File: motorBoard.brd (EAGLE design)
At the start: 97.8 x 68.6 mm, 71 parts, among them J1 TE-TERM-BLOCK, J2 TE-TERM-BLOCK

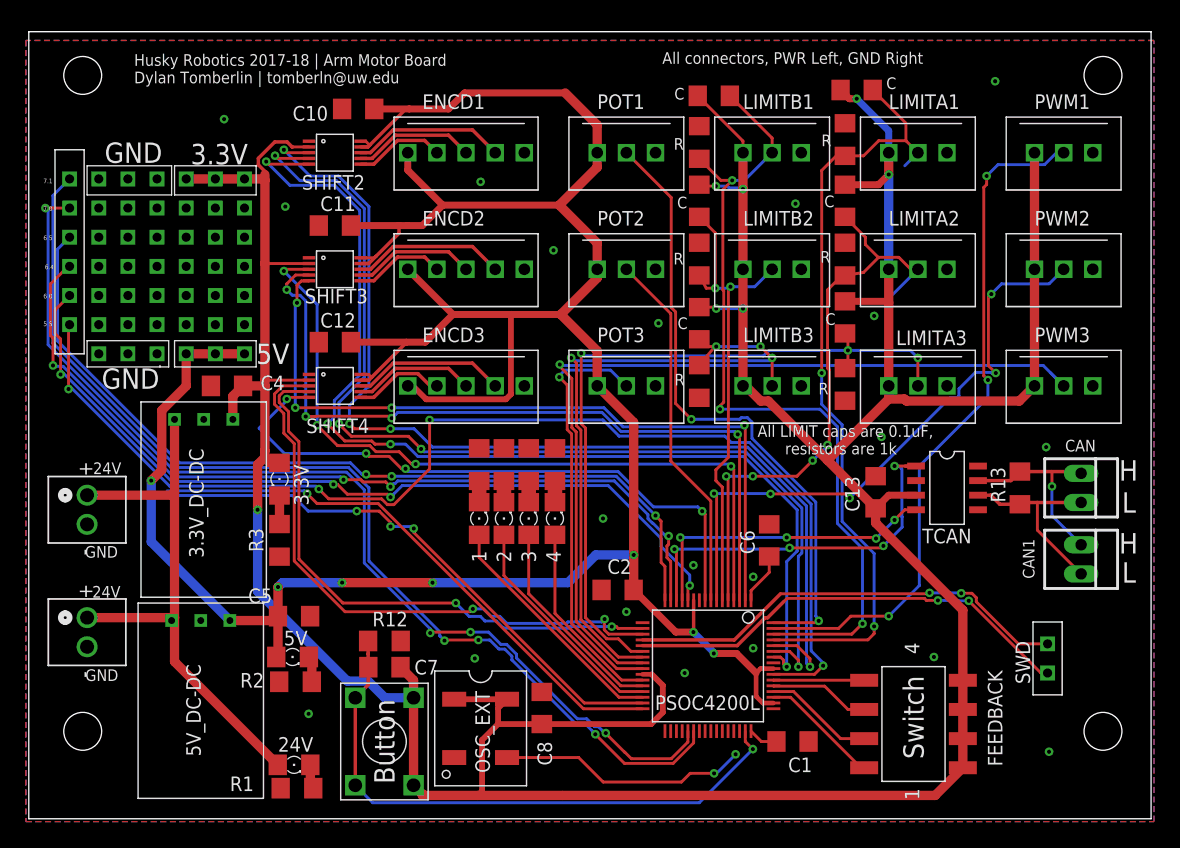
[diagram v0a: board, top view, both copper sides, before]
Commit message: Made changes for Bay Area Circuits DFM
Re-Zipped
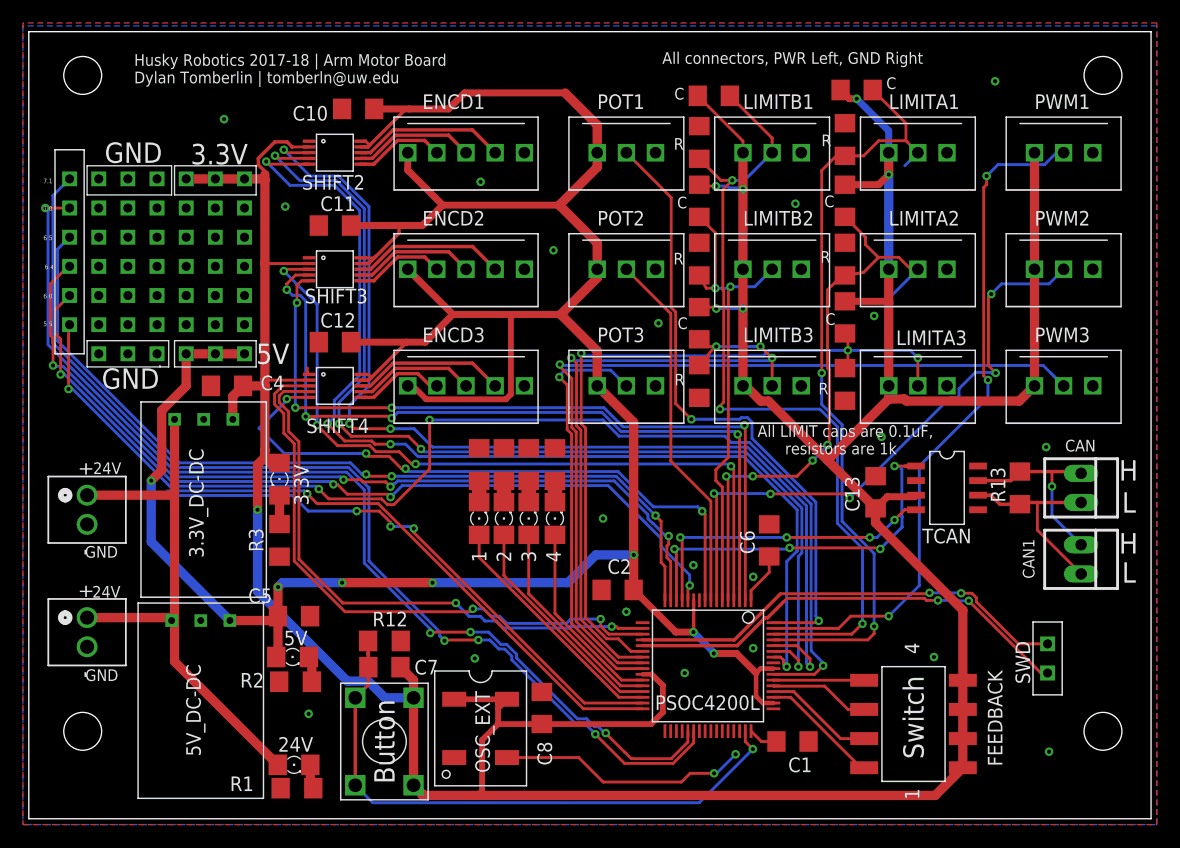
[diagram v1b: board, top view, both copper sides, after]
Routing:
- net GNDA: track 0.00 -> 0.63 mm
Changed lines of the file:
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@@
 <setting verticaltext="up"/>
 </settings>
-<grid distance="0.000000123031" unitdist="inch" unit="inch" style="lines" multiple="1" display="no" altdistance="0.125" altunitdist="inch" altunit="inch"/>
+<grid distance="10" unitdist="mil" unit="mil" style="dots" multiple="1" display="yes" altdistance="0.125" altunitdist="inch" altunit="inch"/>
 <layers>
 <layer number="1" name="Top" color="4" fill="1" visible="yes" active="yes"/>
@@
 <via x="56.7744" y="24.511" extent="1-16" drill="0.35"/>
 <via x="75.438" y="26.035" extent="1-16" drill="0.35"/>
-<wire x1="73.822940625" y1="24.419940625" x2="75.438" y2="26.035" width="0.254" layer="16"/>
 <wire x1="75.438" y1="26.035" x2="76.327" y2="26.924" width="0.254" layer="1"/>
 <wire x1="76.327" y1="26.924" x2="77.31" y2="26.924" width="0.254" layer="1"/>
 <wire x1="56.7744" y1="24.511" x2="66.04" y2="24.511" width="0.254" layer="16"/>
 <via x="66.04" y="24.511" extent="1-16" drill="0.35"/>
-<wire x1="73.73188125" y1="24.511" x2="66.04" y2="24.511" width="0.254" layer="1"/>
-<wire x1="73.73188125" y1="24.511" x2="73.822940625" y2="24.419940625" width="0.254" layer="1"/>
-<via x="73.822940625" y="24.419940625" extent="1-16" drill="0.35"/>
+<wire x1="75.438" y1="26.035" x2="73.914" y2="24.511" width="0.254" layer="16"/>
+<wire x1="73.914" y1="24.511" x2="73.279" y2="24.511" width="0.254" layer="16"/>
+<via x="73.279" y="24.511" extent="1-16" drill="0.35"/>
+<wire x1="73.279" y1="24.511" x2="66.04" y2="24.511" width="0.254" layer="1"/>
 </signal>
 <signal name="CANTX">
@@
 <wire x1="66.1868" y1="23.495" x2="66.294" y2="23.6022" width="0.254" layer="16"/>
 <via x="66.294" y="23.6022" extent="1-16" drill="0.35"/>
-<wire x1="66.294" y1="23.6022" x2="74.29044375" y2="23.6022" width="0.254" layer="1"/>
-<wire x1="74.29044375" y1="23.6022" x2="74.4655625" y2="23.77731875" width="0.254" layer="1"/>
-<via x="74.4655625" y="23.77731875" extent="1-16" drill="0.35"/>
-<wire x1="74.4655625" y1="23.77731875" x2="76.0956" y2="25.40735625" width="0.254" layer="16"/>
 <wire x1="76.0956" y1="25.40735625" x2="76.0956" y2="26.3073875" width="0.254" layer="16"/>
 <wire x1="76.327" y1="30.734" x2="77.31" y2="30.734" width="0.254" layer="1"/>
@@
 <via x="75.438" y="30.734" extent="1-16" drill="0.35"/>
 <wire x1="75.438" y1="30.734" x2="77.31" y2="30.734" width="0.254" layer="1"/>
+<wire x1="66.294" y1="23.6022" x2="74.1017875" y2="23.6022" width="0.254" layer="1"/>
+<wire x1="74.1017875" y1="23.6022" x2="74.19285" y2="23.5111375" width="0.254" layer="1"/>
+<via x="74.19285" y="23.5111375" extent="1-16" drill="0.35"/>
+<wire x1="74.19285" y1="23.5111375" x2="76.08906875" y2="25.40735625" width="0.254" layer="16"/>
+<wire x1="76.08906875" y1="25.40735625" x2="76.0956" y2="25.40735625" width="0.254" layer="16"/>
 </signal>
 <signal name="+5V">
@@
 <via x="52.07" y="18.034" extent="1-16" drill="0.35"/>
 <via x="24.384" y="9.144" extent="1-16" drill="0.35"/>
-<polygon width="0.1524" layer="1">
-<vertex x="-0.254" y="-0.254"/>
-<vertex x="98.044" y="-0.254"/>
-<vertex x="98.044" y="67.818"/>
-<vertex x="-0.254" y="67.818"/>
-</polygon>
-<polygon width="0.1524" layer="16">
-<vertex x="-0.254" y="-0.254"/>
-<vertex x="98.044" y="-0.254"/>
-<vertex x="98.044" y="67.818"/>
-<vertex x="-0.254" y="67.818"/>
-</polygon>
 <contactref element="J1" pad="R"/>
 <contactref element="J2" pad="R"/>
@@
 <contactref element="R14" pad="1"/>
 <contactref element="R15" pad="1"/>
+<wire x1="24.42" y1="38.719" x2="24.2703375" y2="38.8686625" width="0.254" layer="1"/>
+<wire x1="24.2703375" y1="38.8686625" x2="24.2703375" y2="39.28686875" width="0.254" layer="1"/>
+<polygon width="0.1524" layer="1">
+<vertex x="-0.508" y="-0.508"/>
+<vertex x="98.298" y="-0.508"/>
+<vertex x="98.298" y="69.342"/>
+<vertex x="-0.508" y="69.342"/>
+</polygon>
+<polygon width="0.1524" layer="16">
+<vertex x="-0.254" y="-0.508"/>
+<vertex x="98.298" y="-0.508"/>
+<vertex x="98.298" y="69.088"/>
+<vertex x="-0.508" y="69.088"/>
+<vertex x="-0.508" y="-0.508"/>
+</polygon>
 </signal>
 <signal name="+3V3">
@@
 <wire x1="54.2817375" y1="12.585" x2="55.245" y2="11.6217375" width="0.508" layer="1"/>
 <wire x1="53.482" y1="12.585" x2="54.2817375" y2="12.585" width="0.4064" layer="1"/>
-<wire x1="73.787" y1="27.048" x2="74.933" y2="28.194" width="0.6096" layer="1"/>
-<wire x1="74.933" y1="28.194" x2="77.31" y2="28.194" width="0.6096" layer="1"/>
 <wire x1="22.995" y1="58.539" x2="24.42" y2="58.539" width="0.254" layer="1"/>
 <wire x1="20.5640125" y1="31.4860125" x2="20.5640125" y2="32.05911875" width="0.8128" layer="1"/>
@@
 <wire x1="71.12" y1="45.088" x2="74.8" y2="45.088" width="0.6096" layer="1"/>
 <wire x1="74.8" y1="45.088" x2="74.93" y2="44.958" width="0.6096" layer="1"/>
+<wire x1="73.787" y1="27.048" x2="74.8003625" y2="28.0613625" width="0.6096" layer="1"/>
+<wire x1="77.1773625" y1="28.0613625" x2="77.31" y2="28.194" width="0.6096" layer="1"/>
+<wire x1="74.8003625" y1="28.0613625" x2="77.1773625" y2="28.0613625" width="0.6096" layer="1"/>
 </signal>
 <signal name="SEL_SW3">
@@
 <wire x1="22.117275" y1="37.719" x2="21.415" y2="37.016725" width="0.254" layer="1"/>
 <wire x1="21.415" y1="37.016725" x2="21.415" y2="36.115475" width="0.254" layer="1"/>
-<via x="50.1723625" y="17.4002" extent="1-16" drill="0.35"/>
-<wire x1="50.5276125" y1="16.085" x2="50.1424" y2="16.4702125" width="0.254" layer="1"/>
-<wire x1="50.1424" y1="16.4702125" x2="50.1424" y2="17.0149875" width="0.254" layer="1"/>
-<wire x1="50.1424" y1="17.0149875" x2="50.1723625" y2="17.04495" width="0.254" layer="1"/>
-<wire x1="50.1723625" y1="17.04495" x2="50.1723625" y2="17.4002" width="0.254" layer="1"/>
 <wire x1="53.482" y1="16.085" x2="50.5276125" y2="16.085" width="0.254" layer="1"/>
-<wire x1="50.1723625" y1="17.4002" x2="49.9211625" y2="17.149" width="0.254" layer="16"/>
-<wire x1="49.9211625" y1="17.149" x2="46.96825" y2="17.149" width="0.254" layer="16"/>
-<wire x1="46.96825" y1="17.149" x2="46.8433625" y2="17.0241125" width="0.254" layer="16"/>
 <wire x1="46.8433625" y1="17.0241125" x2="41.6498875" y2="17.0241125" width="0.254" layer="16"/>
+<wire x1="49.827371875" y1="16.785240625" x2="49.827371875" y2="17.4002" width="0.254" layer="1"/>
+<via x="49.827371875" y="17.4002" extent="1-16" drill="0.35"/>
+<wire x1="49.827371875" y1="17.4002" x2="47.21945" y2="17.4002" width="0.254" layer="16"/>
+<wire x1="50.5276125" y1="16.085" x2="49.827371875" y2="16.785240625" width="0.254" layer="1"/>
+<wire x1="47.21945" y1="17.4002" x2="46.8433625" y2="17.0241125" width="0.254" layer="16"/>
 </signal>
 <signal name="MOTOR4LIMB">
